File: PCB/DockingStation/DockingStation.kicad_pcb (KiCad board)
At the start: 4 copper layers, 147.2 x 63.2 mm, 256 parts, among them CN1 DSUB-15-HD_Socket_Horizontal_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, CN2 FDC_Connector, CN4 DSUB-25_Socket_Horizontal_P2.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, CN5 DSUB-9_Pins_Horizontal_P2.77x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, CN6 PS2 Connector, CN7 PS2 Connector, CN8 BarrelJack_Horizontal_PC110, J1 25-1MP_P0.5mm_Horizontal, J2 25-1MP_P0.5mm_Horizontal, J3 25-1MP_P0.5mm_Horizontal, J4 25-1MP_P0.5mm_Horizontal, Q1 3P4J, Q2 8C, U1 74VHCT244, U2 DNP (LT1237CS), U3 DS14C535MSA, U4 DNP

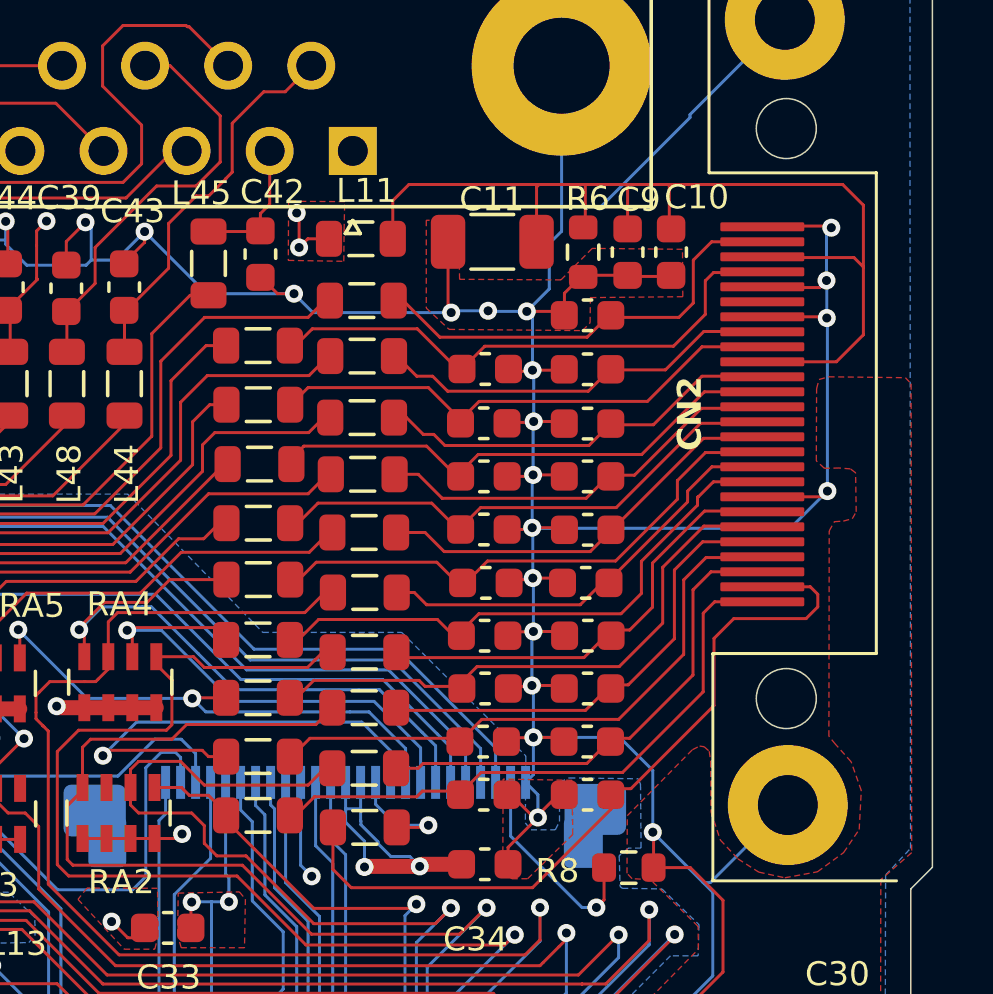
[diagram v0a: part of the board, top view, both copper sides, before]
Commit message: Add files via upload
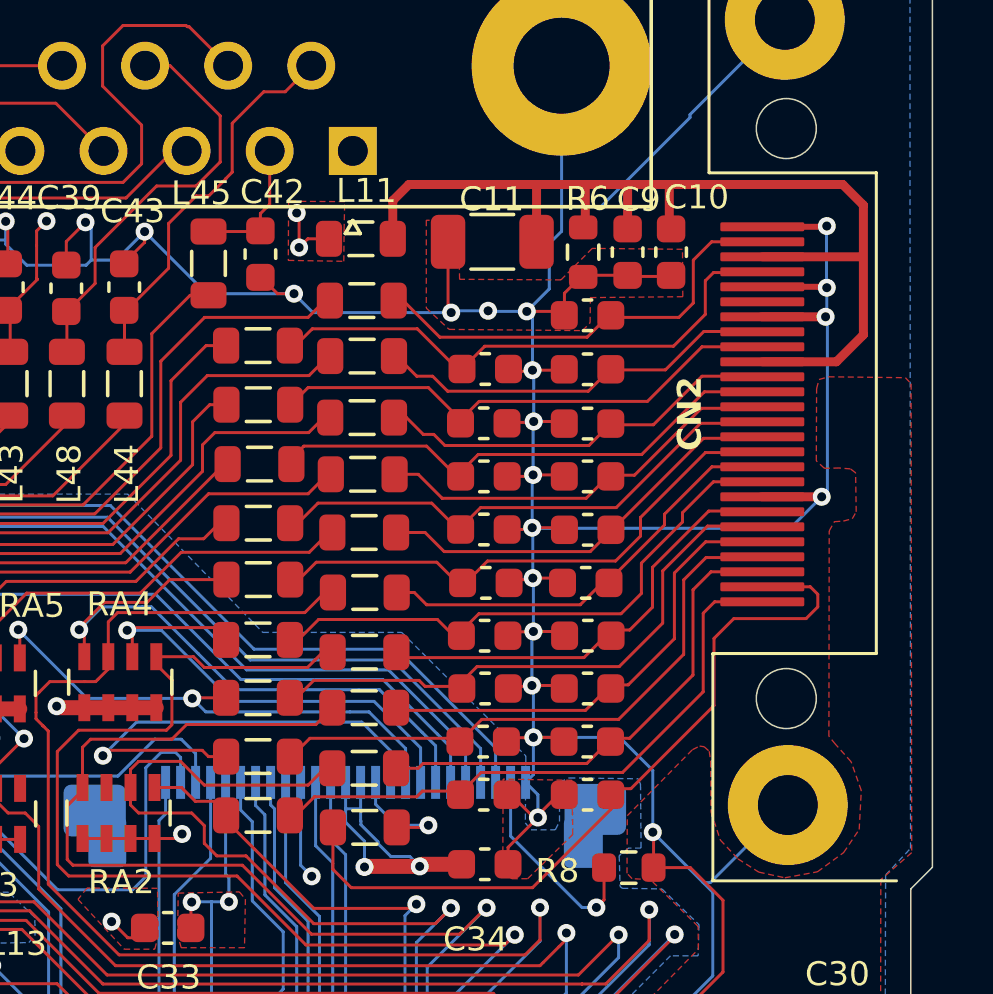
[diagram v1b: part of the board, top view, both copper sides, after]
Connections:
- net FDC_DRATE0_MEDIA_ID0 renamed FDC_DRATE0
- net FDC_DRATE1_MEDIA_ID1 renamed FDC_DRATE1
- net FDC_DS0# renamed FDD_DRSEL
- net FDC_MTR0# renamed FDD_MOTEN
- net J13_90_PC110 renamed FDD_Bowman
- net J13_92_PC110 renamed FDD_Pluto4
- net J13_95_PC110 renamed FDD_Pluto3
- net J13_97_PC110 renamed FDD_Pluto2
- net J13_98_PC110 renamed FDD_Pluto1
- C13 pad 1: J13_90_PC110_L31 -> FDD_Bowman_L31
- C17 pad 2: J13_92_PC110_L29 -> FDD_Pluto4_L29
- C23 pad 2: J13_95_PC110_L26 -> FDD_Pluto3_L26
- C24 pad 1: FDC_MTR0#_L16 -> FDD_MOTEN_L16
- C25 pad 2: FDC_DRATE0_MEDIA_ID0_L25 -> FDC_DRATE0_L25
- C26 pad 1: FDC_DS0#_L16 -> FDD_DRSEL_L16
- C27 pad 2: J13_97_PC110_L24 -> FDD_Pluto2_L24
- C29 pad 2: J13_98_PC110_L23 -> FDD_Pluto1_L23
- C30 pad 1: FDC_DRATE1_MEDIA_ID1_L13 -> FDC_DRATE1_L13
- CN2 pad 10: FDD_PWR_L11 -> GND
- CN2 pad 11: FDC_DS0#_L16 -> FDD_Pluto4_L29
- CN2 pad 12: FDC_DRATE0_MEDIA_ID0_L25 -> FDC_RDATA#_L30
- CN2 pad 13: FDC_MTR0#_L16 -> FDD_Bowman_L31
- CN2 pad 14: J13_95_PC110_L26 -> FDC_DRATE1_L13
- CN2 pad 15: FDC_DIR#_L17 -> FDD_Pluto1_L23
- CN2 pad 16: FDC_STEP#_L27 -> CN2_6
- CN2 pad 17: FDC_WDATA#_L18 -> FDC_INDEX#_L14
- CN2 pad 18: FDC_WGATE#_L28 -> FDD_PWR_L11
- CN2 pad 19: GND -> FDC_DRATE0_L25
- CN2 pad 2: FDC_DRATE1_MEDIA_ID1_L13 -> FDD_PWR_L11
- CN2 pad 20: FDC_TRK0_L19 -> FDD_Pluto3_L26
- CN2 pad 21: J13_92_PC110_L29 -> FDC_STEP#_L27
- CN2 pad 22: FDC_WRTPRT#_L20 -> FDC_WGATE#_L28
- CN2 pad 23: FDC_RDATA#_L30 -> FDC_TRK0_L19
- CN2 pad 24: FDC_HDSEL#_L21 -> FDC_WRTPRT#_L20
- CN2 pad 25: J13_90_PC110_L31 -> FDC_HDSEL#_L21
- CN2 pad 3: FDD_PWR_L11 -> GND
- CN2 pad 4: J13_98_PC110_L23 -> GND
- CN2 pad 5: GND -> FDD_Pluto2_L24
- CN2 pad 6: CN2_6 -> FDD_DRSEL_L16
- CN2 pad 7: GND -> FDD_MOTEN_L16
- CN2 pad 8: FDC_INDEX#_L14 -> FDC_DIR#_L17
- CN2 pad 9: J13_97_PC110_L24 -> FDC_WDATA#_L18
- L13 pad 2: FDC_DRATE1_MEDIA_ID1_L13 -> FDC_DRATE1_L13
- L15 pad 2: FDC_DS0#_L16 -> FDD_DRSEL_L16
- L16 pad 2: FDC_MTR0#_L16 -> FDD_MOTEN_L16
- L23 pad 2: J13_98_PC110_L23 -> FDD_Pluto1_L23
- L24 pad 2: J13_97_PC110_L24 -> FDD_Pluto2_L24
- L25 pad 2: FDC_DRATE0_MEDIA_ID0_L25 -> FDC_DRATE0_L25
- L26 pad 2: J13_95_PC110_L26 -> FDD_Pluto3_L26
- L29 pad 2: J13_92_PC110_L29 -> FDD_Pluto4_L29
- L31 pad 1: J13_90_PC110_L31 -> FDD_Bowman_L31
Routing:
- net J13_90_PC110_L31: track 25.8 -> 0.00 mm
- net FDD_Bowman_L31: track 0.00 -> 25.8 mm
- net J13_92_PC110_L29: track 19.4 -> 0.00 mm
- net FDD_Pluto4_L29: track 0.00 -> 19.4 mm
- net J13_98_PC110_L23: track 18.6 -> 0.00 mm
- net FDD_Pluto1_L23: track 0.00 -> 18.6 mm
- net J13_95_PC110_L26: track 17.9 -> 0.00 mm
- net FDD_Pluto3_L26: track 0.00 -> 17.9 mm
- net FDC_DRATE0_MEDIA_ID0_L25: track 17.7 -> 0.00 mm
- net FDC_DRATE0_L25: track 0.00 -> 17.7 mm
- net J13_97_PC110_L24: track 17.5 -> 0.00 mm
- net FDD_Pluto2_L24: track 0.00 -> 17.5 mm
- net FDC_DRATE1_MEDIA_ID1_L13: track 14.9 -> 0.00 mm
- net FDC_DRATE1_L13: track 0.00 -> 14.9 mm
- net FDD_MOTEN_L16: track 0.00 -> 13.8 mm
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
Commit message: Add files via upload
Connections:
- net J13_41_PC110 renamed Modem_RSRVD2
- net J13_42_PC110 renamed Modem_RSRVD1
- net J13_52_PC110 renamed MN192_VPDA#
- net J13_58_PC110 renamed MN195_S11_BUF
- net J13_59_PC110 renamed MN195_ADCK#
- net J13_60_PC110 renamed MN195_IRQ1#
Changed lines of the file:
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@@
 	(net 70 "M38_P16_R80_PC110")
 	(net 71 "M38_P67")
-	(net 72 "J13_60_PC110")
-	(net 73 "J13_59_PC110")
-	(net 74 "J13_58_PC110")
-	(net 75 "J13_52_PC110")
+	(net 72 "MN195_IRQ1#")
+	(net 73 "MN195_ADCK#")
+	(net 74 "MN195_S11_BUF")
+	(net 75 "MN192_VPDA#")
 	(net 76 "J13_49_PC110")
-	(net 77 "J13_41_PC110")
-	(net 78 "J13_42_PC110")
+	(net 77 "Modem_RSRVD2")
+	(net 78 "Modem_RSRVD1")
 	(net 79 "J13_43_PC110")
 	(net 80 "J13_37_PC110")
@@
 			(size 0.3 1.1)
 			(layers "B.Cu" "B.Mask" "B.Paste")
-			(net 72 "J13_60_PC110")
+			(net 72 "MN195_IRQ1#")
 		)
 		(pad "17" smd rect
@@
 			(size 0.3 1.1)
 			(layers "B.Cu" "B.Mask" "B.Paste")
-			(net 73 "J13_59_PC110")
+			(net 73 "MN195_ADCK#")
 		)
 		(pad "18" smd rect
@@
 			(size 0.3 1.1)
 			(layers "B.Cu" "B.Mask" "B.Paste")
-			(net 74 "J13_58_PC110")
+			(net 74 "MN195_S11_BUF")
 		)
 		(pad "19" smd rect
@@
 			(size 0.3 1.1)
 			(layers "B.Cu" "B.Mask" "B.Paste")
-			(net 75 "J13_52_PC110")
+			(net 75 "MN192_VPDA#")
 		)
 		(pad "25" smd rect
@@
 			(size 0.3 1.1)
 			(layers "B.Cu" "B.Mask" "B.Paste")
-			(net 77 "J13_41_PC110")
+			(net 77 "Modem_RSRVD2")
 		)
 		(pad "17" smd rect
@@
 			(size 0.3 1.1)
 			(layers "B.Cu" "B.Mask" "B.Paste")
-			(net 78 "J13_42_PC110")
+			(net 78 "Modem_RSRVD1")
 		)
 		(pad "18" smd rect

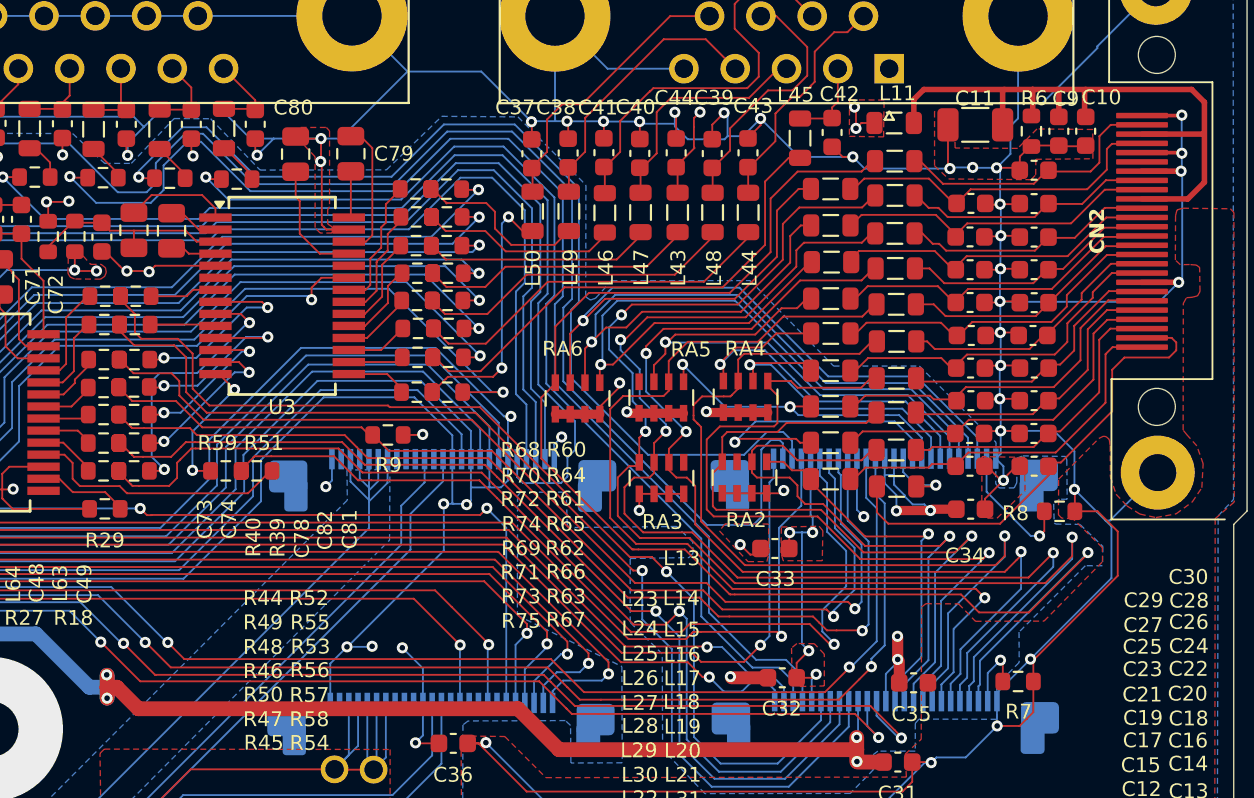
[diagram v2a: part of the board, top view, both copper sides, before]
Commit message: Add files via upload
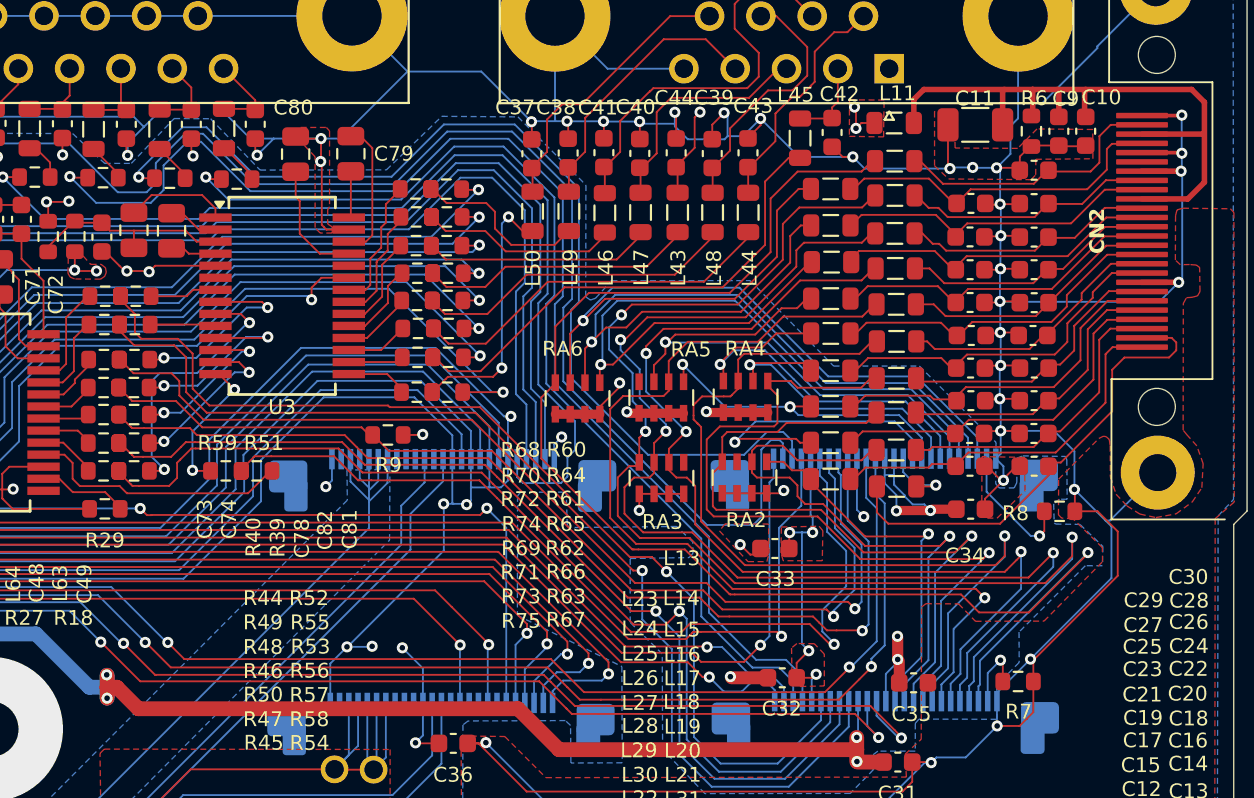
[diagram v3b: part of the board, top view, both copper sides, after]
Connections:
- net J13_2_PC110 renamed Pluto_Dock1_PC110
- net J13_99_PC110 renamed Pluto_Dock2_PC110
- RA2 pad 1: RA2 -> FDD_PWR
- RA2 pad 2: RA2 -> FDD_PWR
- RA2 pad 3: RA2 -> FDD_PWR
- RA2 pad 4: RA2 -> FDD_PWR
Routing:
- net FDD_PWR: track 92.8 -> 96.1 mm, vias 10 -> 11
- net RA2: track 3.38 -> 0.00 mm, vias 1 -> 0

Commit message: Add files via upload
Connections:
- CN5 pad 1: CN5_1 -> DCD2#
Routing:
- net DCD2#: track 4.92 -> 16.1 mm
